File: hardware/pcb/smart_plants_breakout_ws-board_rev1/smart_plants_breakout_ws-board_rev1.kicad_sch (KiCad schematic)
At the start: 27 parts, among them J1 Breakout, J10 Pump, J11 I2C D6-powered, J2 Breakout, J3 I2C, J4 USB-C Power, J5 I2C D3-powered, J6 I2C, J7 Battery, J8 Board Power, J9 Moisture Sensor, Q1 IRLZ14, SW1 Power Switch, U1 XIAO-ESP32-C6

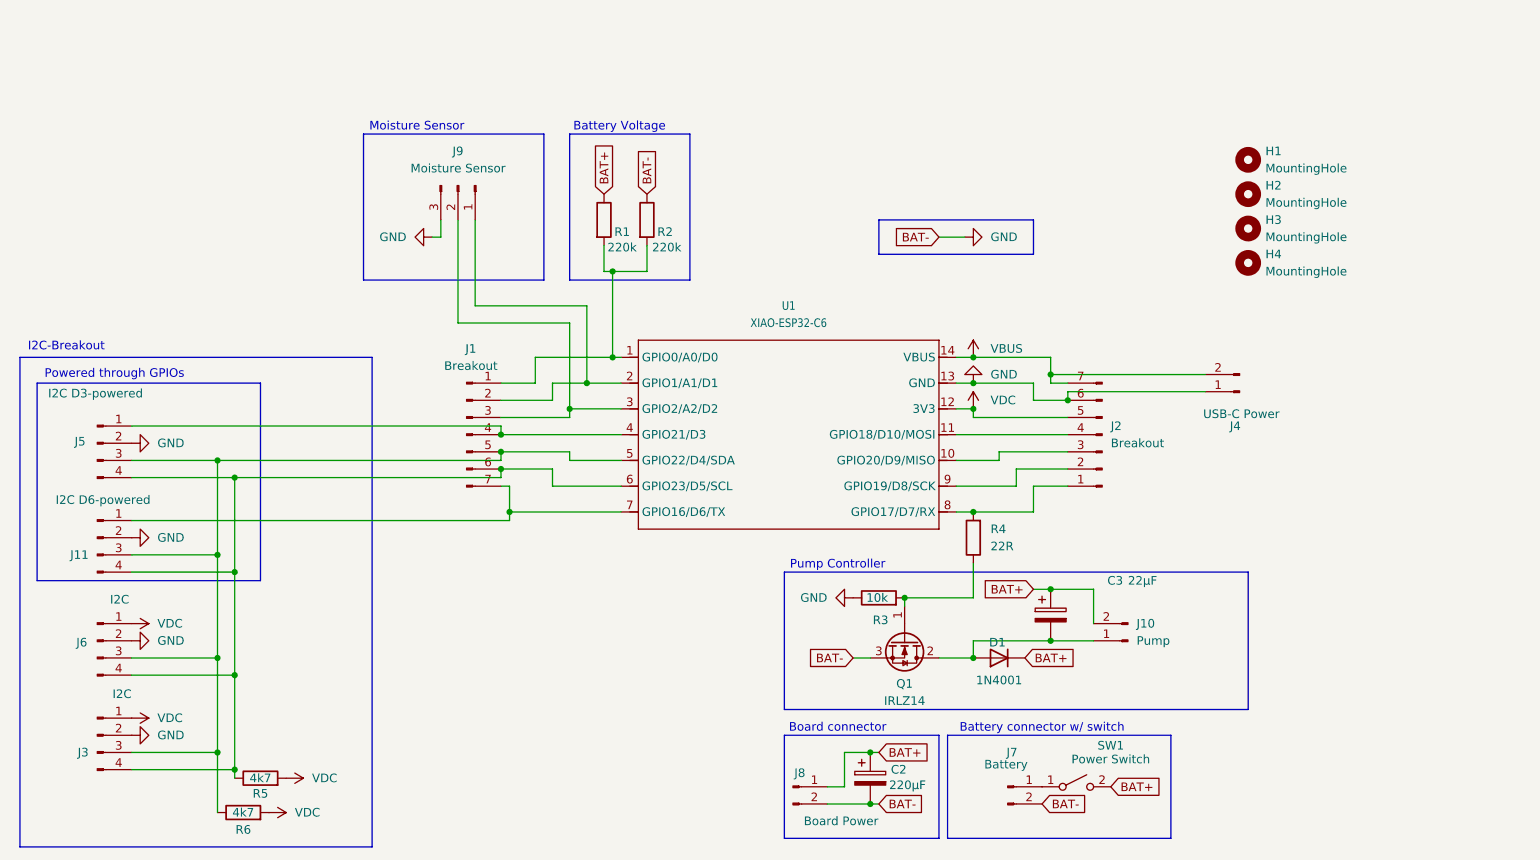
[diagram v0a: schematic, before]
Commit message: Added PCB
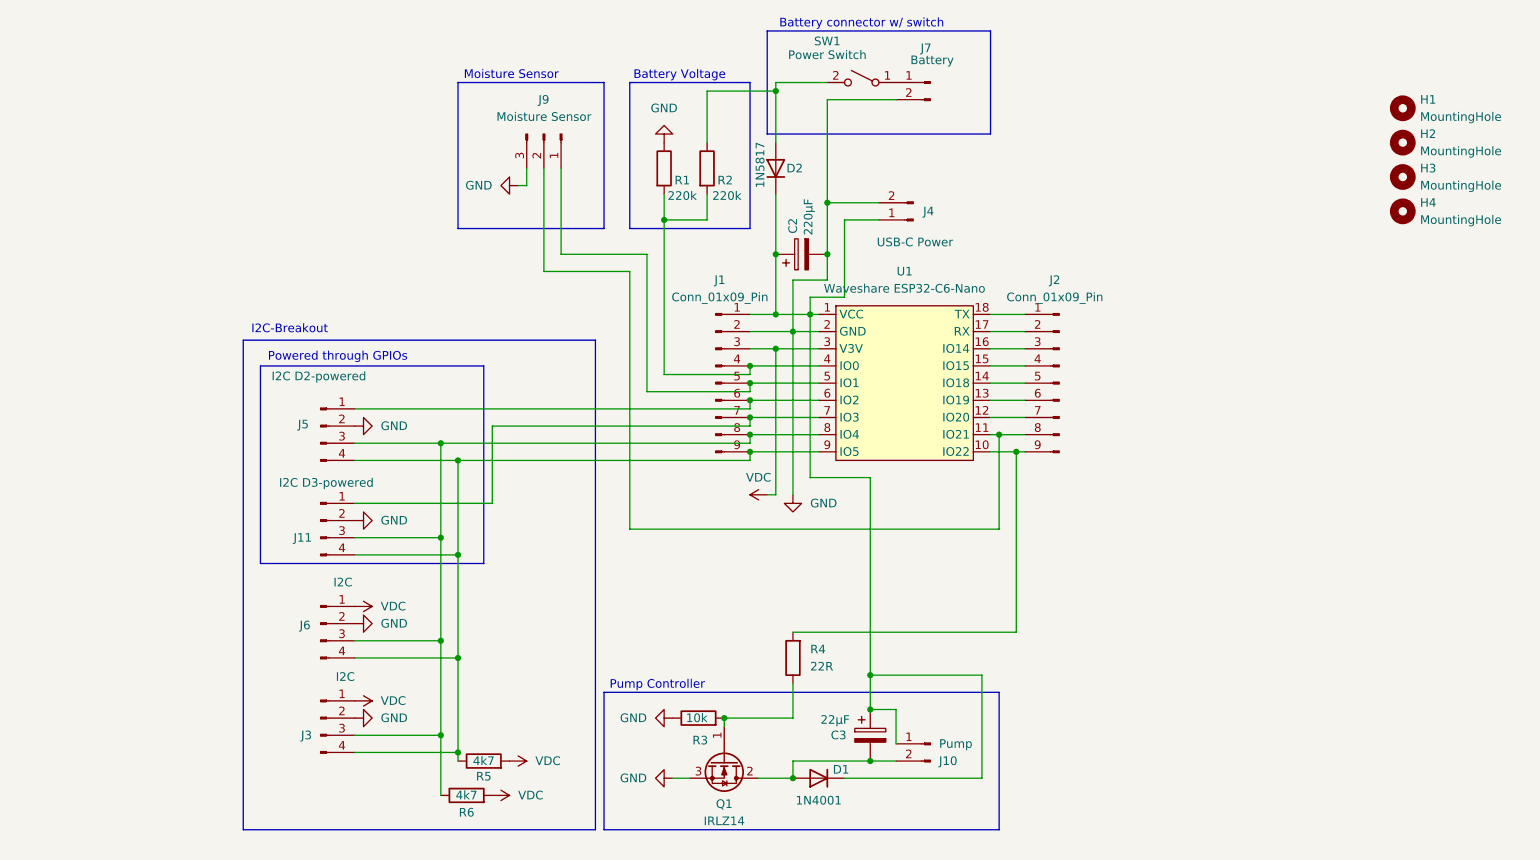
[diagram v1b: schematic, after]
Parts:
- removed J1, J2: Breakout, Connector_PinHeader_2.54mm:PinHeader_1x07_P2.54mm_Vertical, symbol Connector:Conn_01x07_Pin
- removed J8: Board Power, Connector_JST:JST_XH_B2B-XH-A_1x02_P2.50mm_Vertical, symbol Connector:Conn_01x02_Pin
- removed U1: XIAO-ESP32-C6, XIAO ESP32 Family:XIAO-ESP32C6-DIP, symbol XIAO ESP Family:XIAO_ESP32-C6-DIP
- added D2: 1N5817, Diode_THT:D_DO-41_SOD81_P10.16mm_Horizontal, symbol Diode:1N4001
- added J1, J2: Conn_01x09_Pin, Connector_PinSocket_2.54mm:PinSocket_1x09_P2.54mm_Vertical, symbol Connector:Conn_01x09_Pin
- added U1: Waveshare ESP32-C6-Nano, ws-esp32c6:Waveshare-ESP32-C6-Zero, symbol ws-esp32-c6:Waveshare-ESP32-C6-Zero
- J11: value I2C D6-powered -> I2C D3-powered
- J5: value I2C D3-powered -> I2C D2-powered
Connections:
- net VBUS is gone; now on net GND: J4.2 (Pin_2)
- net GND: now also R1.1, J1.2 (Pin_2), U1.2 (GND); no longer J4.1 (Pin_1), R2.1
- net VDC: now also J1.3 (Pin_3), U1.3 (V3V)
- net at R1.2, R2.2: now also J1.4 (Pin_4), U1.4 (IO0)
- net at J11.3 (Pin_3), J3.3 (Pin_3), J5.3 (Pin_3)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: now also J1.8 (Pin_8), U1.8 (IO4)
- net at C3.2, D1.2 (A), Q1.2 (D): now also J10.2 (Pin_2); no longer J10.1 (Pin_1)
- net at J11.4 (Pin_4), J3.4 (Pin_4), J5.4 (Pin_4)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: now also J1.9 (Pin_9), U1.9 (IO5)
- net at R4.2: now also J2.9 (Pin_9), U1.10 (IO22)
- net at J9.1 (Pin_1): now also J1.5 (Pin_5), U1.5 (IO1)
- net at J9.2 (Pin_2): now also J2.8 (Pin_8), U1.11 (IO21)
- net at J11.1 (Pin_1): now also J1.7 (Pin_7), U1.7 (IO3)
- net at J5.1 (Pin_1): now also J1.6 (Pin_6), U1.6 (IO2)
- net BAT+: no longer names the net of C2.1, C3.1, D1.1 (K)
- net BAT+: now also J10.1 (Pin_1), J4.1 (Pin_1), D2.1 (K), J1.1 (Pin_1), U1.1 (VCC); no longer J10.2 (Pin_2), R1.1, SW1.2 (B)
- new net: D2.2 (A), R2.1, SW1.2 (B)
- new net: J2.1 (Pin_1), U1.18 (TX)
- new net: J2.2 (Pin_2), U1.17 (RX)
- new net: J2.3 (Pin_3), U1.16 (IO14)
- new net: J2.4 (Pin_4), U1.15 (IO15)
- new net: J2.5 (Pin_5), U1.14 (IO18)
- new net: J2.6 (Pin_6), U1.13 (IO19)
- new net: J2.7 (Pin_7), U1.12 (IO20)
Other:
- note removed: "Board connector"
- title: Smart Plants Breakout PCB -> (none)
- moved on the sheet: C2, C3, D1, H1, H2, H3, H4, J10, J11, J3, J4, J5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

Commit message: WS PCB bug fixes
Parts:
- J4: footprint Connector_JST:JST_XH_B2B-XH-A_1x02_P2.50mm_Vertical -> Connector_JST:JST_PH_B2B-PH-K_1x02_P2.00mm_Vertical
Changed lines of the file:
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@@
 			)
 		)
-		(property "Footprint" "Connector_JST:JST_XH_B2B-XH-A_1x02_P2.50mm_Vertical"
+		(property "Footprint" "Connector_JST:JST_PH_B2B-PH-K_1x02_P2.00mm_Vertical"
 			(at 160.02 53.34 0)
 			(effects
